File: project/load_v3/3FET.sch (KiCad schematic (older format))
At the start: 24 parts, among them P14 IN, P15 OUT, Q6 Q_NMOS_GDS, Q7 Q_NMOS_GDS, Q8 Q_NMOS_GDS, U8 LM324

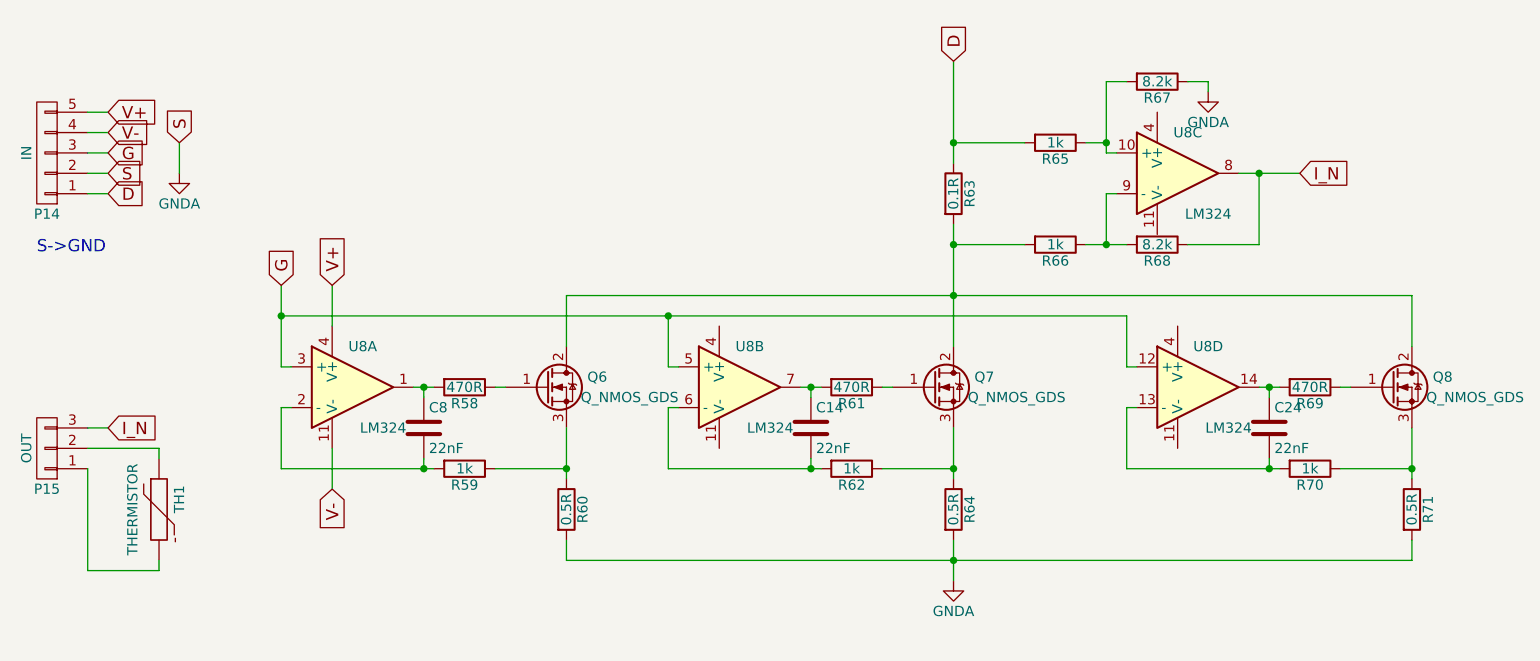
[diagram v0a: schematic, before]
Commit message: a
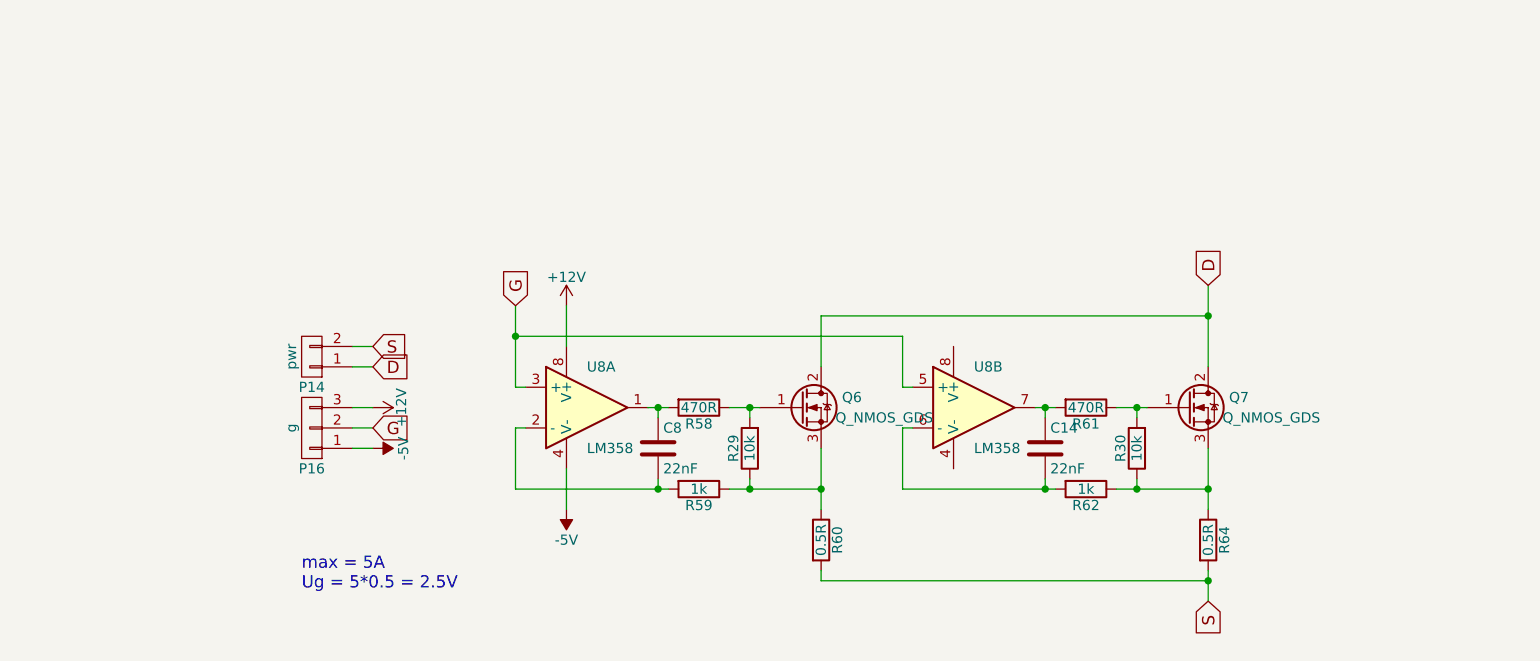
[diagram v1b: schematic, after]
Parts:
- removed C24: 22nF, symbol C
- removed P14: IN, symbol CONN_01X05
- removed P15: OUT, symbol CONN_01X03
- removed Q8: Q_NMOS_GDS, symbol Q_NMOS_GDS
- removed R63: 0.1R, symbol R
- removed R65, R66, R70: 1k, symbol R
- removed R67, R68: 8.2k, symbol R
- removed R69: 470R, symbol R
- removed R71: 0.5R, symbol R
- removed TH1: THERMISTOR, symbol THERMISTOR
- removed U8: LM324, symbol LM324
- added P14: pwr, Connectors_Phoenix:PhoenixContact_MCV-G_02x5.08mm_Vertical, symbol CONN_01X02
- added P16: g, Connectors:XH2.54-3P, symbol CONN_01X03
- added R29, R30: 10k, Resistors_THT:Resistor_Horizontal_RM7mm, symbol R
- added U8: LM358, Housings_DIP:DIP-8_W7.62mm_LongPads, symbol LM358
- C14, C8: footprint (none) -> Capacitors_THT:C_Disc_D3_P2.5
- Q6, Q7: footprint (none) -> TO_SOT_Packages_THT:TO-247_Vertical_Neutral123
- R58, R59, R61, R62: footprint (none) -> Resistors_THT:Resistor_Horizontal_RM7mm
- R60, R64: footprint (none) -> Resistors_THT:Resistor_Vertical_RM7.5mm
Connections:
- net D: now also Q6.2 (D), Q7.2 (D), P14.1 (P1)
- net G: now also P16.2 (P2), U8.3 (+), U8.5 (+)
- net at Q6.3 (S), R59.1, R60.1: now also R29.1
- net at Q7.3 (S), R62.1, R64.1: now also R30.1
- net at Q6.1 (G), R58.1: now also R29.2
- net at C8.1, R58.2: now also U8.1
- net at Q7.1 (G), R61.1: now also R30.2
- net at C14.1, R61.2: now also U8.7
- net at C8.2, R59.2: now also U8.2 (-)
- net at C14.2, R62.2: now also U8.6 (-)
- net GNDA renamed S
- net S: now also P14.2 (P2)
- new net +12V: P16.3 (P3), U8.8 (V+)
- new net -5V: P16.1 (P1), U8.4 (V-)
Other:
- note added: "max = 5A\nUg = 5*0.5 = 2.5V"
- note removed: "S->GND"
- moved on the sheet: C14, C8, Q6, Q7, R58, R59, R60, R61, R62, R64
